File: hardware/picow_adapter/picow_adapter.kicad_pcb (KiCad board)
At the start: 2 copper layers, 33 x 63.5 mm, 2 parts, among them Q1 DMG2305UX

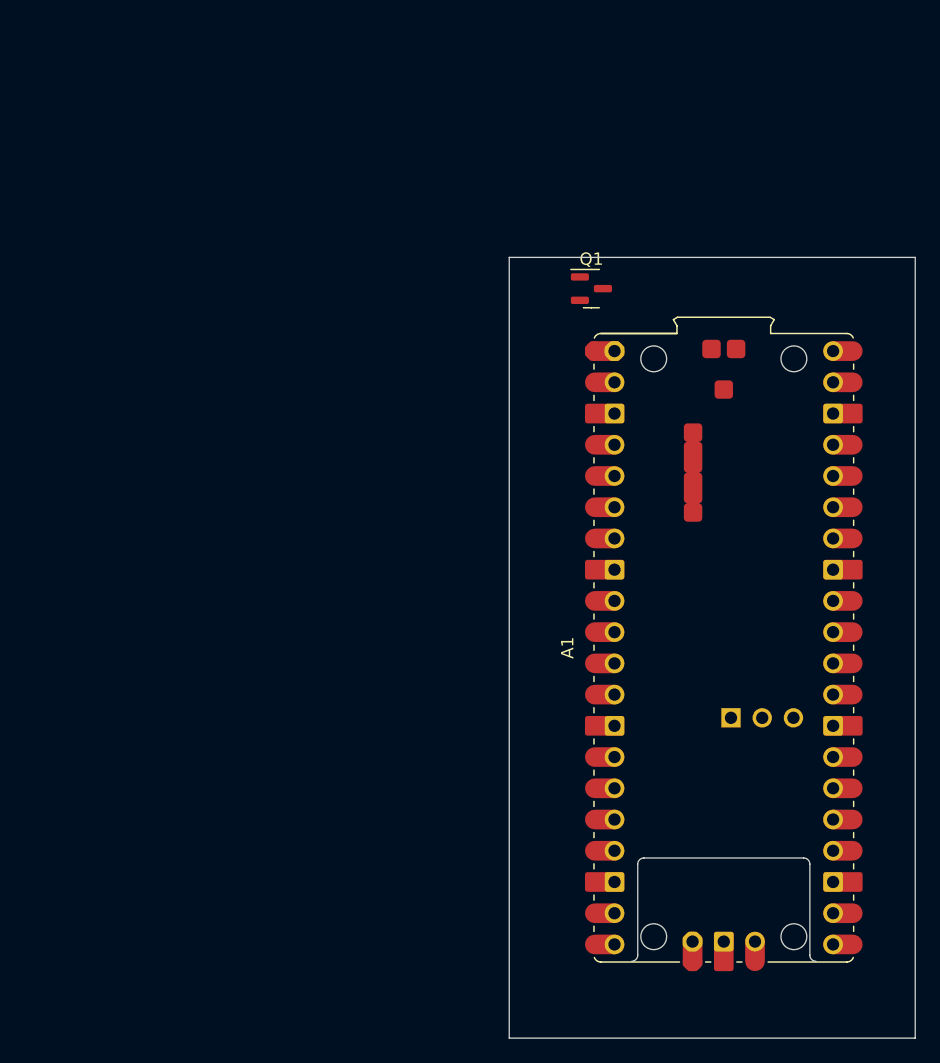
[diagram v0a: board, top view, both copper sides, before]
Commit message: update
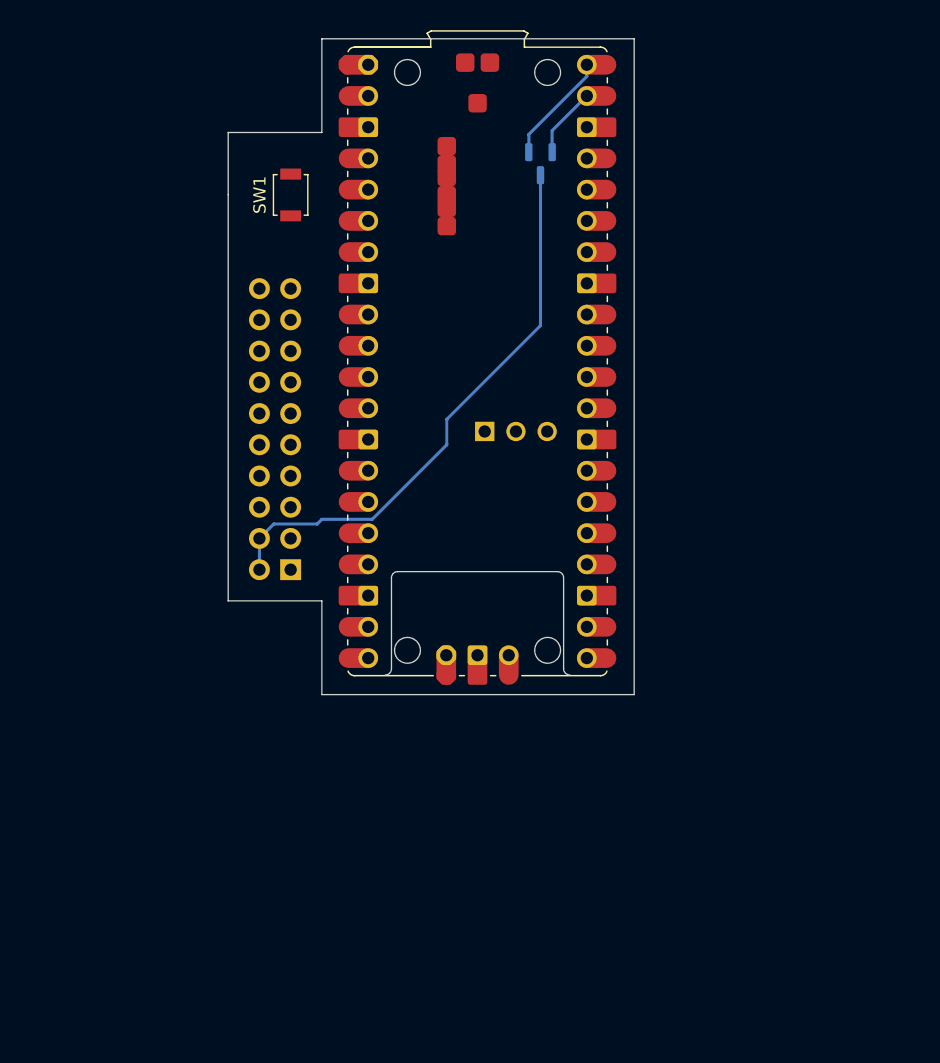
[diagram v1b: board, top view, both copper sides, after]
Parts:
- added J1: Sensorclock, Connector_PinSocket_2.54mm:PinSocket_2x10_P2.54mm_Vertical, B.Cu at (68.6, 83.8)
- added SW1: SW_Push, Button_Switch_SMD:SW_SPST_B3U-1000P, F.Cu at (68.6, 53.3)
- Q1: moved to B.Cu
- moved A1 30.7 mm to (74.9, 42.8)
- moved Q1 11.0 mm to (88.9, 50.8), turned to -90 degrees
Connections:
- A1 pad 24: unconnected-(A1-GPIO18-Pad24) -> /SPI0_SCK
- A1 pad 25: unconnected-(A1-GPIO19-Pad25) -> /SPI0_TX
- A1 pad 30: unconnected-(A1-RUN-Pad30) -> /RESET
- A1 pad 6: unconnected-(A1-GPIO4-Pad6) -> /I2C0_SDA
- A1 pad 7: unconnected-(A1-GPIO5-Pad7) -> /I2C0_SCL
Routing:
- net +5V: track 0.00 -> 46.0 mm
- net Net-(A1-VBUS): track 0.00 -> 9.07 mm
- net Net-(A1-VSYS): track 0.00 -> 5.74 mm
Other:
- board size 33 x 63.5 mm -> 33 x 53.3 mm

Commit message: update
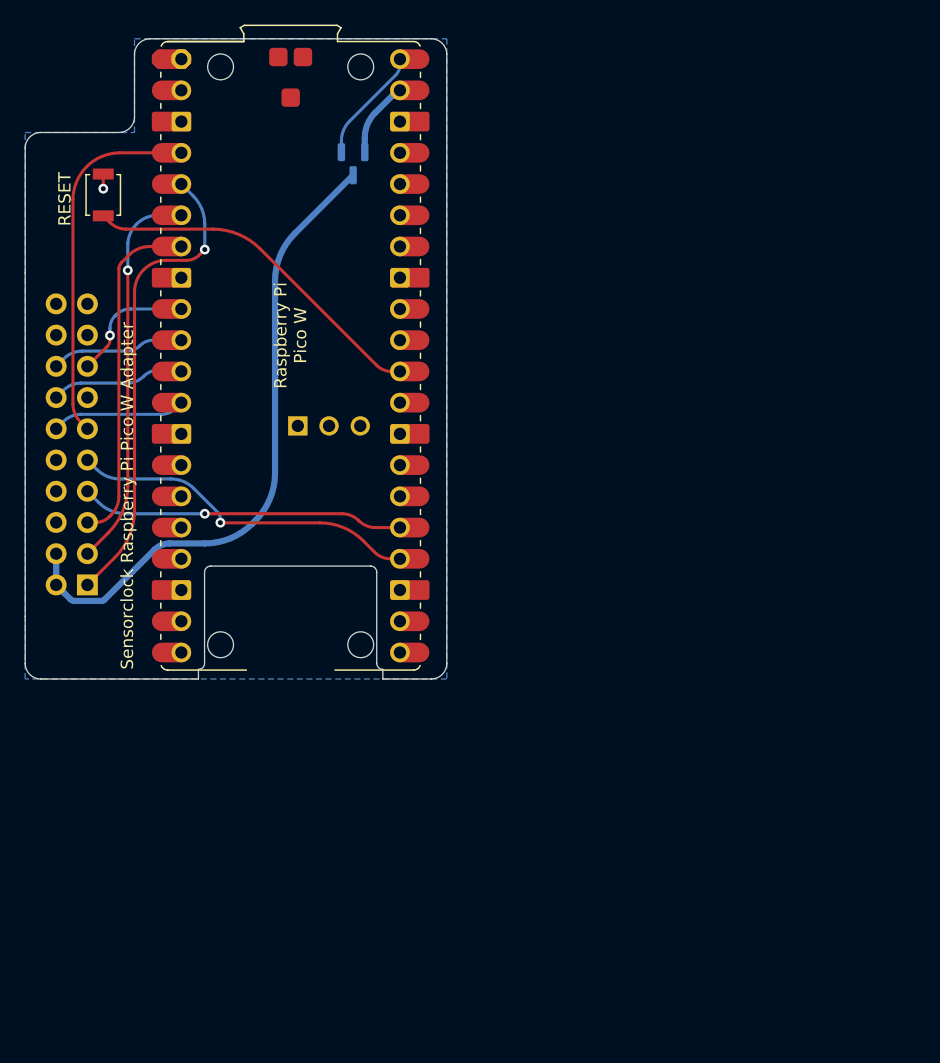
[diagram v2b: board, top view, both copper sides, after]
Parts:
- moved J1 16.6 mm to (52.0, 85.1)
- moved Q1 15.2 mm to (73.7, 50.8)
- moved SW1 15.2 mm to (53.3, 53.3)
- moved A1 15.2 mm to (59.7, 42.3)
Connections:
- A1 pad 10: unconnected-(A1-GPIO7-Pad10) -> /S1_B
- A1 pad 11: unconnected-(A1-GPIO8-Pad11) -> /S1_S
- A1 pad 12: unconnected-(A1-GPIO9-Pad12) -> /TSL2561_INT
- A1 pad 4: unconnected-(A1-GPIO2-Pad4) -> /HEATER_ENABLE
- A1 pad 5: unconnected-(A1-GPIO3-Pad5) -> /~{SHDN_3V3}
- A1 pad 9: unconnected-(A1-GPIO6-Pad9) -> /S1_A
- J1 pad 13: /DS3231_INT -> unconnected-(J1-Pin_13-Pad13)
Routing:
- net /~{SHDN_3V3}: track 0.00 -> 38.6 mm, vias 0 -> 1
- net /I2C0_SDA: track 0.00 -> 31.9 mm, vias 0 -> 1
- net /HEATER_ENABLE: track 0.00 -> 30.0 mm
- net /RESET: track 0.00 -> 28.9 mm
- net /SPI0_SCK: track 0.00 -> 28.5 mm, vias 0 -> 1
- net /I2C0_SCL: track 0.00 -> 28.1 mm
- net /SPI0_TX: track 0.00 -> 26.3 mm, vias 0 -> 1
- net /TSL2561_INT: track 0.00 -> 10.9 mm
- net /S1_S: track 0.00 -> 10.9 mm
- net /S1_B: track 0.00 -> 10.8 mm
- net /S1_A: track 0.00 -> 10.5 mm, vias 0 -> 1
- net +5V: track 46.0 -> 52.4 mm
- net GND: track 0.00 -> 1.19 mm, vias 0 -> 1
- added copper zone on B.Cu, net GND
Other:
- board size 33 x 53.3 mm -> 34.3 x 52.1 mm
- board text added: "RESET"
- board text added: "Raspberry Pi Pico W"
- board text added: "Sensorclock Raspberry Pi Pico W Adapter"
